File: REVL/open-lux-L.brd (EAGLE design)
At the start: 55.7 x 58.5 mm, 65 parts, among them IC2 MCP73831, IC3 ATMEGA32U4-AU, IC4 MCP1700-33, J1 AYZ0202, Q1 BSS123, Q4 BSS123, T1 FDN340P, T2 FDN340P, X2 USBSMD, X3 8MHz

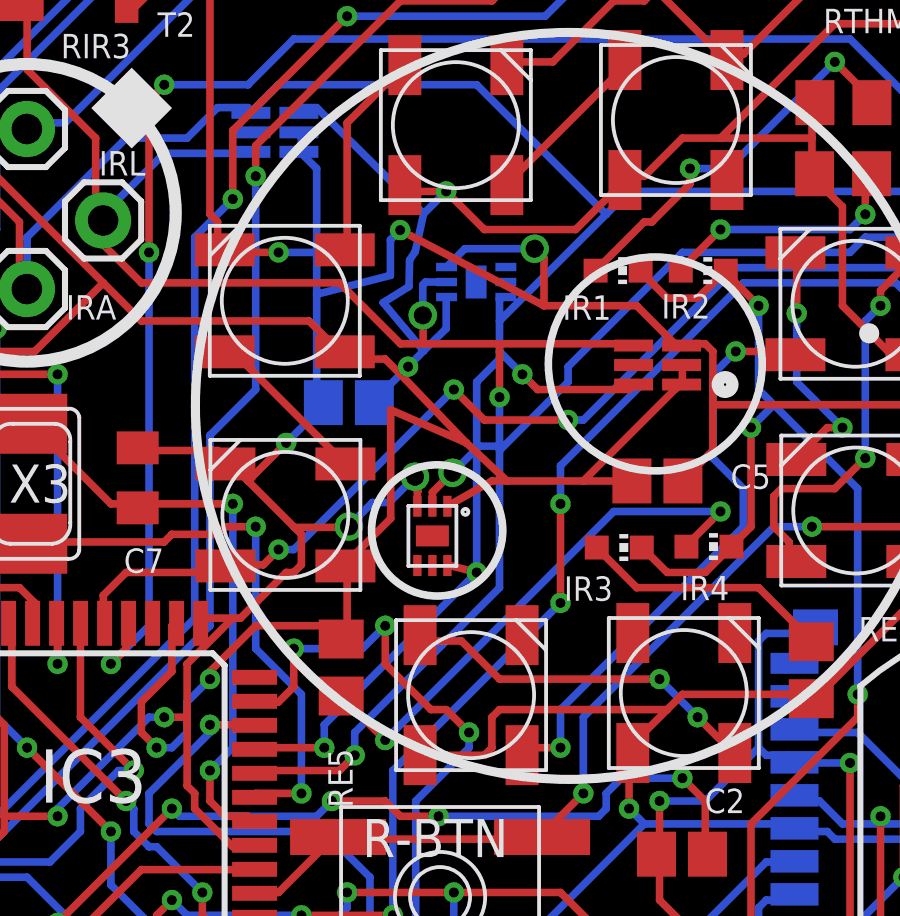
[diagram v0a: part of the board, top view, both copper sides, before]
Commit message: update
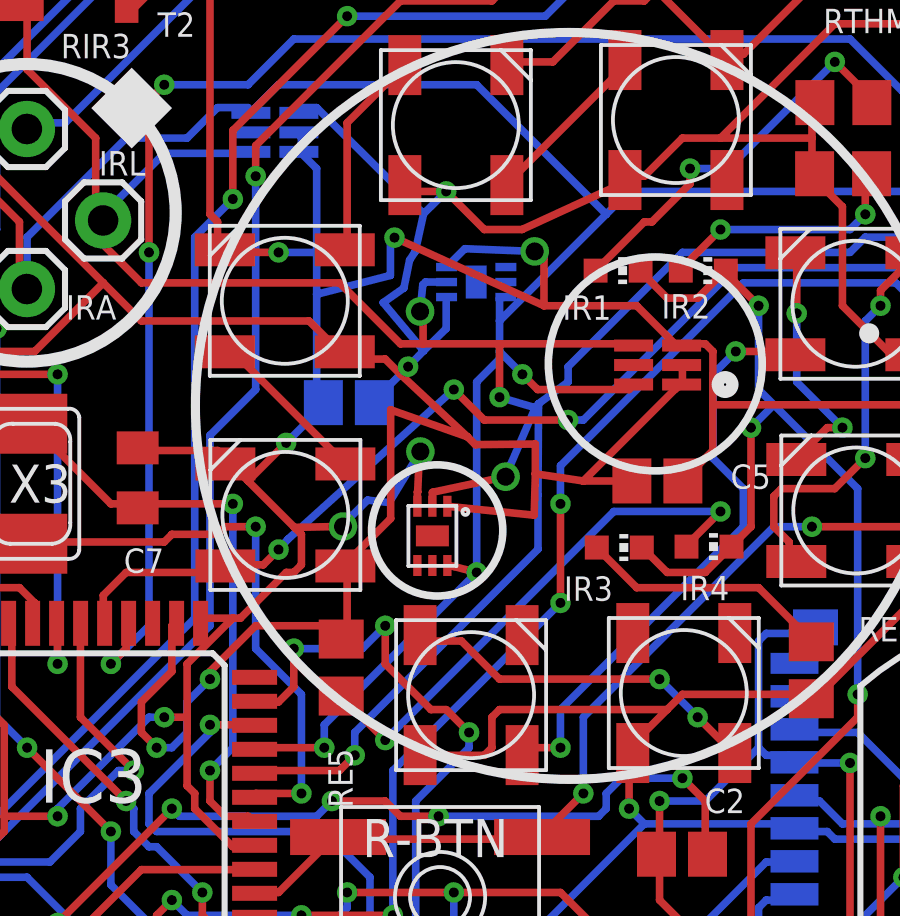
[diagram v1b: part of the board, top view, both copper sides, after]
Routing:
- net VCC: track 354.1 -> 356.2 mm
- net SCL: track 86.0 -> 88.0 mm
- net GND: track 352.1 -> 353.4 mm
